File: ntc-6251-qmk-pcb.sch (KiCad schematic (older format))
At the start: 212 parts, among them J1 USB_B, U1 YAAJ_WeAct_BlackPill_Part_Lik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

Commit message: Created lib for logo
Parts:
- U1: symbol YAAJ_WeAct_BlackPill_Part_Like_SWD_Breakout:YAAJ_WeAct_BlackPill_Part_Like_SWD_Breakout -> ntc-6251-qmk-pcb-rescue:YAAJ_WeAct_BlackPill_Part_Like_SWD_Breakout-YAAJ_WeAct_BlackPill_Part_Like_SWD_Breakout
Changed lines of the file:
@@
 $EndComp
 $Comp
-L YAAJ_WeAct_BlackPill_Part_Like_SWD_Breakout:YAAJ_WeAct_BlackPill_Part_Like_SWD_Breakout U1
+L ntc-6251-qmk-pcb-rescue:YAAJ_WeAct_BlackPill_Part_Like_SWD_Breakout-YAAJ_WeAct_BlackPill_Part_Like_SWD_Breakout U1
 U 1 1 61C1A754
 P 7550 9000

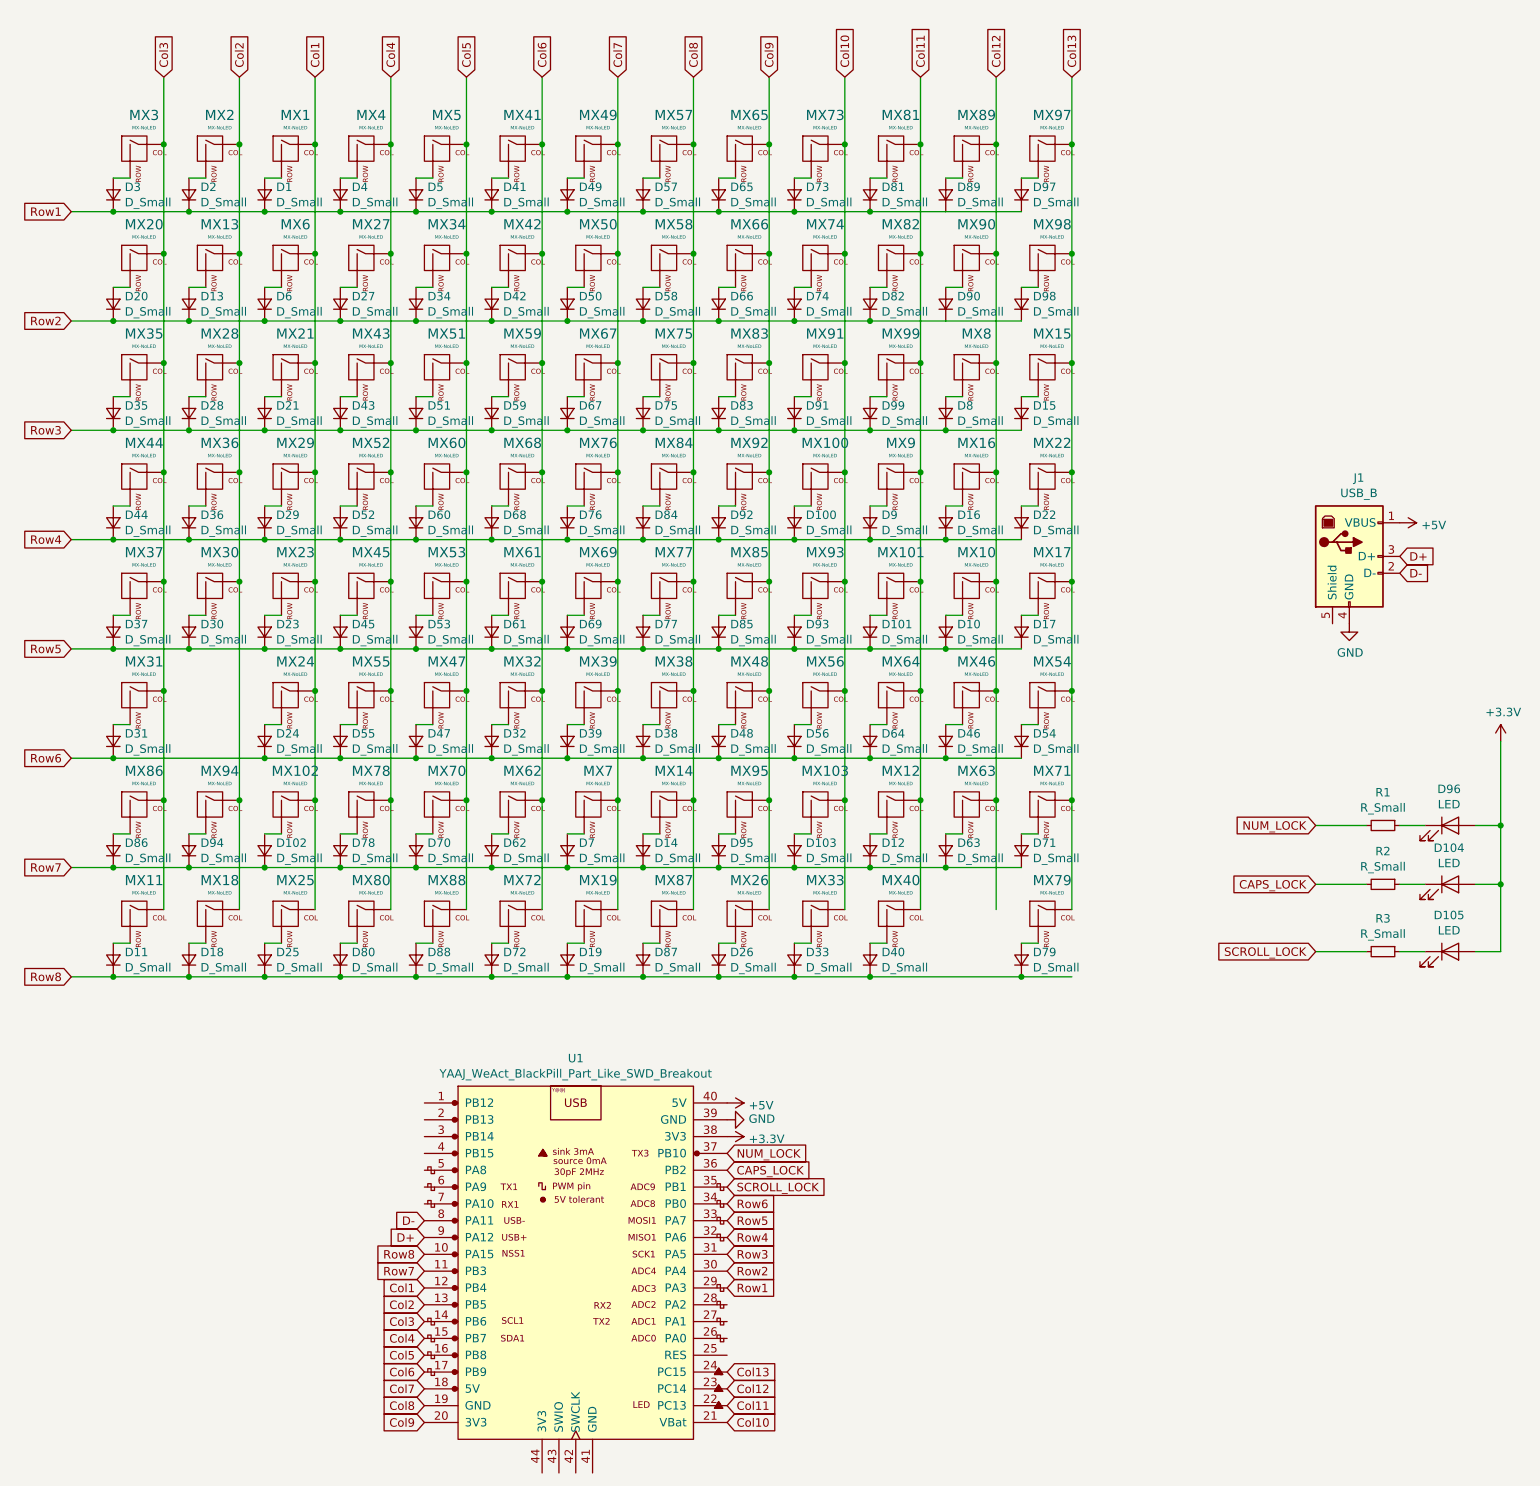
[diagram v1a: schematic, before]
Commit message: Changed connector fixed controller pins, re-routed all traces near controller
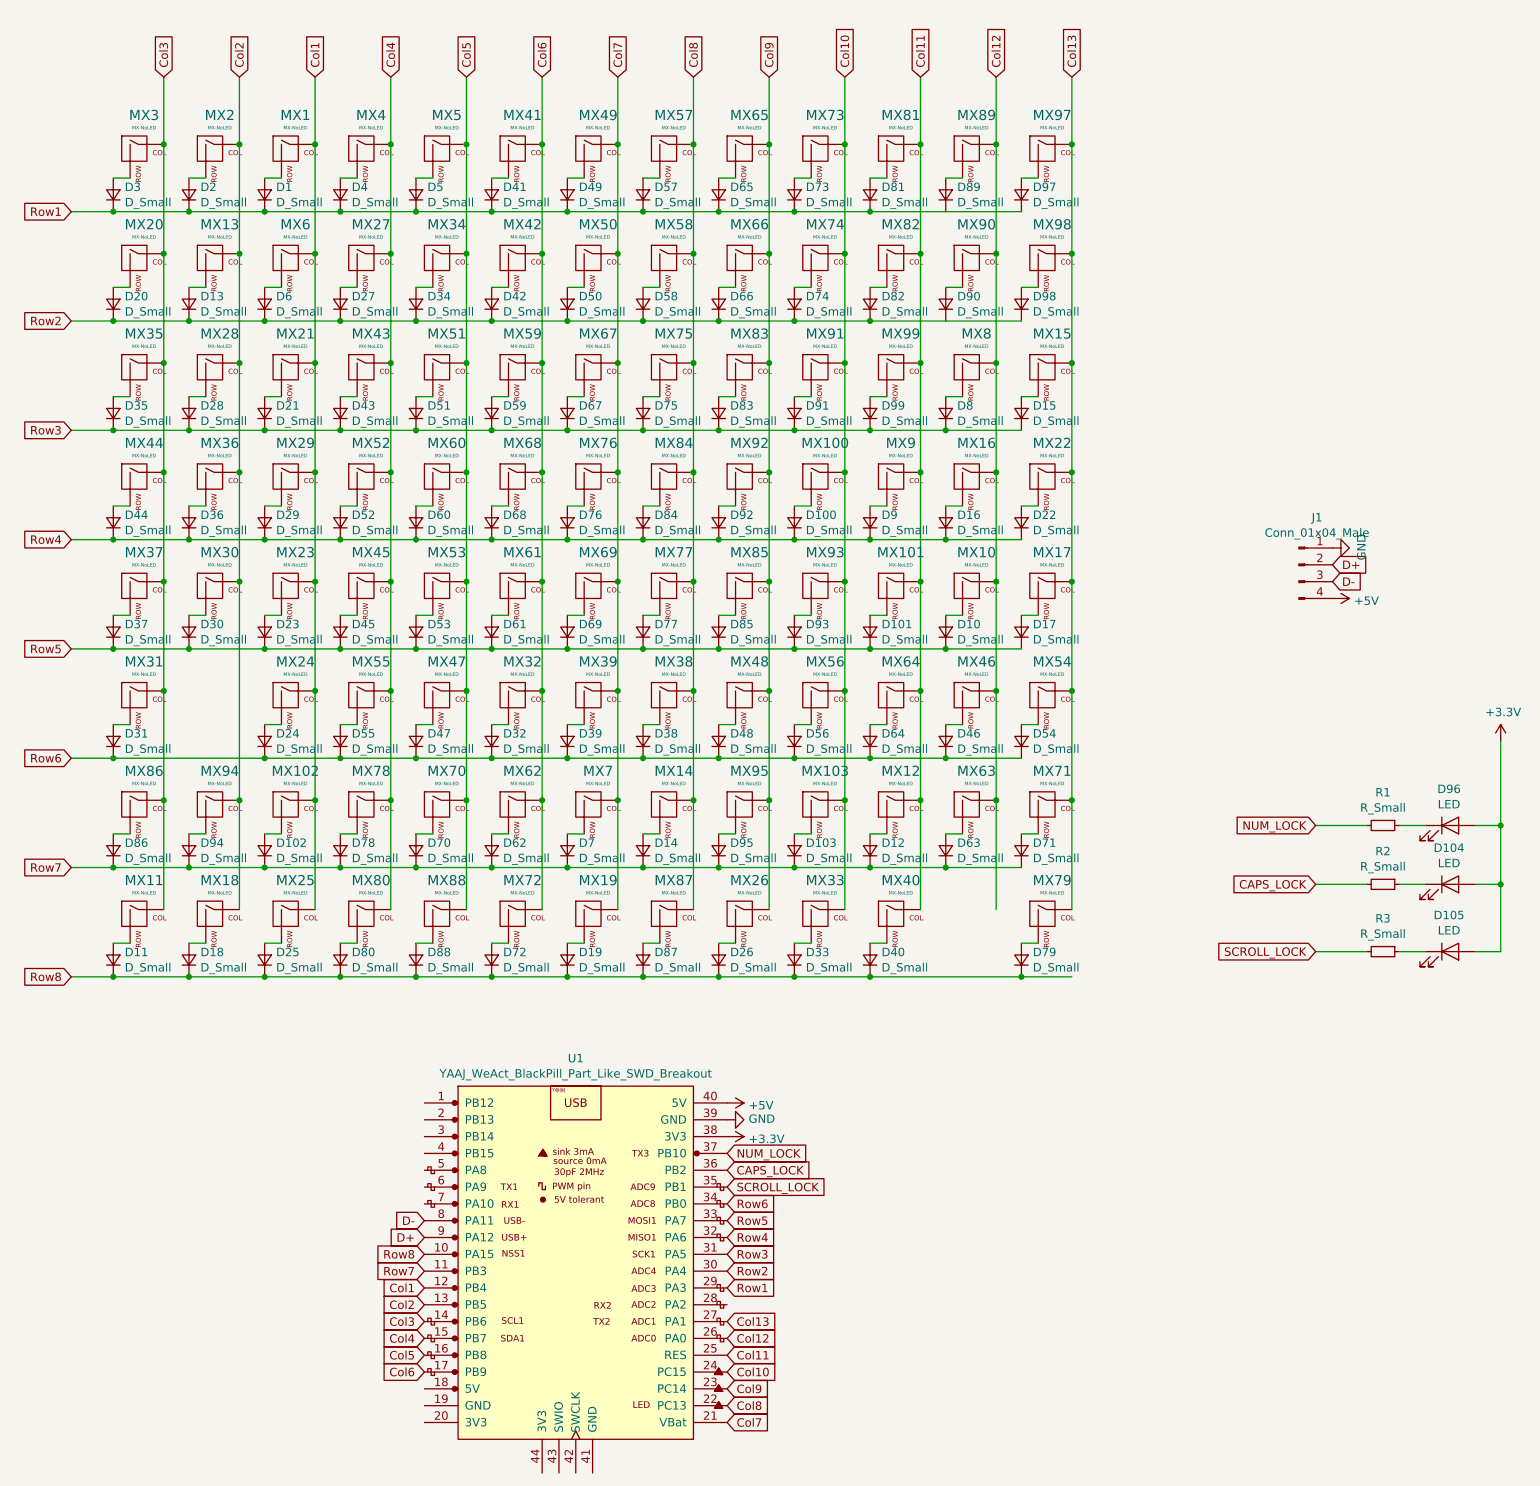
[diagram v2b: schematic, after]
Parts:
- removed J1: USB_B, Connector_USB:USB_B_OST_USB-B1HSxx_Horizontal, symbol Connector:USB_B
- added J1: Conn_01x04_Male, Connector_PinHeader_2.54mm:PinHeader_1x04_P2.54mm_Horizontal, symbol Connector:Conn_01x04_Male
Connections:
- net +5V: now also J1.4 (Pin_4)
- net Col10: now also U1.24 (PC15); no longer U1.21 (VBat)
- net Col11: now also U1.25 (RES); no longer U1.22 (PC13)
- net Col12: now also U1.26 (PA0); no longer U1.23 (PC14)
- net Col13: now also U1.27 (PA1); no longer U1.24 (PC15)
- net Col7: now also U1.21 (VBat); no longer U1.18 (5V)
- net Col8: now also U1.22 (PC13); no longer U1.19 (GND)
- net Col9: now also U1.23 (PC14); no longer U1.20 (3V3)
- net D+: now also J1.2 (Pin_2)
- net D-: now also J1.3 (Pin_3)
- net GND: now also J1.1 (Pin_1)
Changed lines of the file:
@@
 Text GLabel 6650 9700 0    50   Input ~ 0
 Col6
-Text GLabel 6650 9800 0    50   Input ~ 0
+Text GLabel 8450 10000 2    50   Input ~ 0
 Col7
-Text GLabel 6650 9900 0    50   Input ~ 0
+Text GLabel 8450 9900 2    50   Input ~ 0
 Col8
-Text GLabel 6650 10000 0    50   Input ~ 0
+Text GLabel 8450 9800 2    50   Input ~ 0
 Col9
-Text GLabel 8450 10000 2    50   Input ~ 0
+Text GLabel 8450 9700 2    50   Input ~ 0
 Col10
-Text GLabel 8450 9900 2    50   Input ~ 0
+Text GLabel 8450 9600 2    50   Input ~ 0
 Col11
-Text GLabel 8450 9800 2    50   Input ~ 0
+Text GLabel 8450 9500 2    50   Input ~ 0
 Col12
-Text GLabel 8450 9700 2    50   Input ~ 0
+Text GLabel 8450 9400 2    50   Input ~ 0
 Col13
 Wire Wire Line
@@
 $EndComp
 $Comp
-L Connector:USB_B J1
-U 1 1 61E577A0
-P 12150 4850
-F 0 "J1" H 12207 5317 50  0000 C CNN
-F 1 "USB_B" H 12207 5226 50  0000 C CNN
-F 2 "Connector_USB:USB_B_OST_USB-B1HSxx_Horizontal" H 12300 4800 50  0001 C CNN
-F 3 " ~" H 12300 4800 50  0001 C CNN
-	1    12150 4850
-	1    0    0    -1
-$EndComp
-$Comp
 L ntc-6251-qmk-pcb-rescue:YAAJ_WeAct_BlackPill_Part_Like_SWD_Breakout-YAAJ_WeAct_BlackPill_Part_Like_SWD_Breakout U1
 U 1 1 61C1A754
@@
 L power:GND #PWR0101
 U 1 1 61C3454D
-P 12150 5250
-F 0 "#PWR0101" H 12150 5000 50  0001 C CNN
-F 1 "GND" H 12155 5077 50  0000 C CNN
-F 2 "" H 12150 5250 50  0001 C CNN
-F 3 "" H 12150 5250 50  0001 C CNN
-	1    12150 5250
-	1    0    0    -1
+P 12050 4800
+F 0 "#PWR0101" H 12050 4550 50  0001 C CNN
+F 1 "GND" H 12055 4627 50  0000 C CNN
+F 2 "" H 12050 4800 50  0001 C CNN
+F 3 "" H 12050 4800 50  0001 C CNN
+	1    12050 4800
+	0    -1   -1   0
 $EndComp
 $Comp
@@
 	0    1    1    0
 $EndComp
-Text GLabel 12450 4850 2    50   Input ~ 0
+Text GLabel 12050 4900 2    50   Input ~ 0
 D+
-Text GLabel 12450 4950 2    50   Input ~ 0
+Text GLabel 12050 5000 2    50   Input ~ 0
 D-
 Text GLabel 6650 8800 0    50   Input ~ 0
@@
 L power:+5V #PWR0104
 U 1 1 61C4D745
-P 12450 4650
-F 0 "#PWR0104" H 12450 4500 50  0001 C CNN
-F 1 "+5V" V 12465 4778 50  0000 L CNN
-F 2 "" H 12450 4650 50  0001 C CNN
-F 3 "" H 12450 4650 50  0001 C CNN
-	1    12450 4650
+P 12050 5100
+F 0 "#PWR0104" H 12050 4950 50  0001 C CNN
+F 1 "+5V" V 12065 5228 50  0000 L CNN
+F 2 "" H 12050 5100 50  0001 C CNN
+F 3 "" H 12050 5100 50  0001 C CNN
+	1    12050 5100
 	0    1    1    0
 $EndComp
@@
 Wire Wire Line
 	7350 6300 7350 6950
+$Comp
+L Connector:Conn_01x04_Male J1
+U 1 1 61CBF66C
+P 11850 4900
+F 0 "J1" H 11958 5181 50  0000 C CNN
+F 1 "Conn_01x04_Male" H 11958 5090 50  0000 C CNN
+F 2 "Connector_PinHeader_2.54mm:PinHeader_1x04_P2.54mm_Horizontal" H 11850 4900 50  0001 C CNN
+F 3 "~" H 11850 4900 50  0001 C CNN
+	1    11850 4900
+	1    0    0    -1
+$EndComp
 $EndSCHEMATC
